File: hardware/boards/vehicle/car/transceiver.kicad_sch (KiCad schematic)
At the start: 0 parts

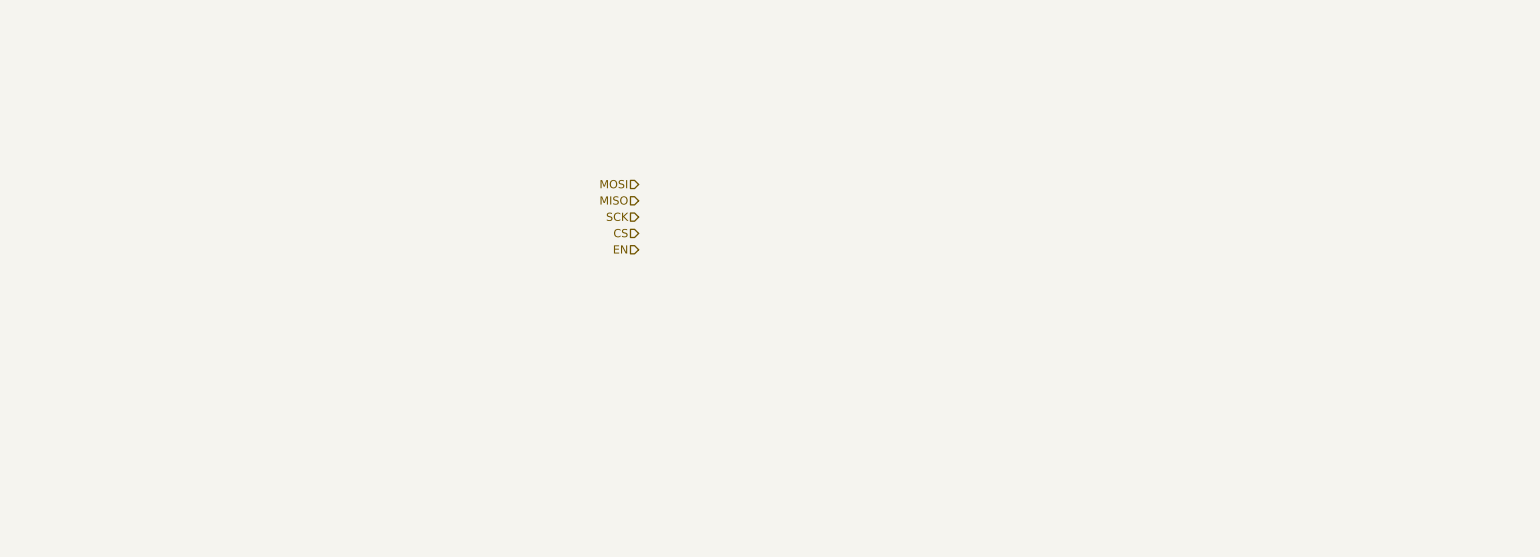
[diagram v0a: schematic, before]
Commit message: car schematic
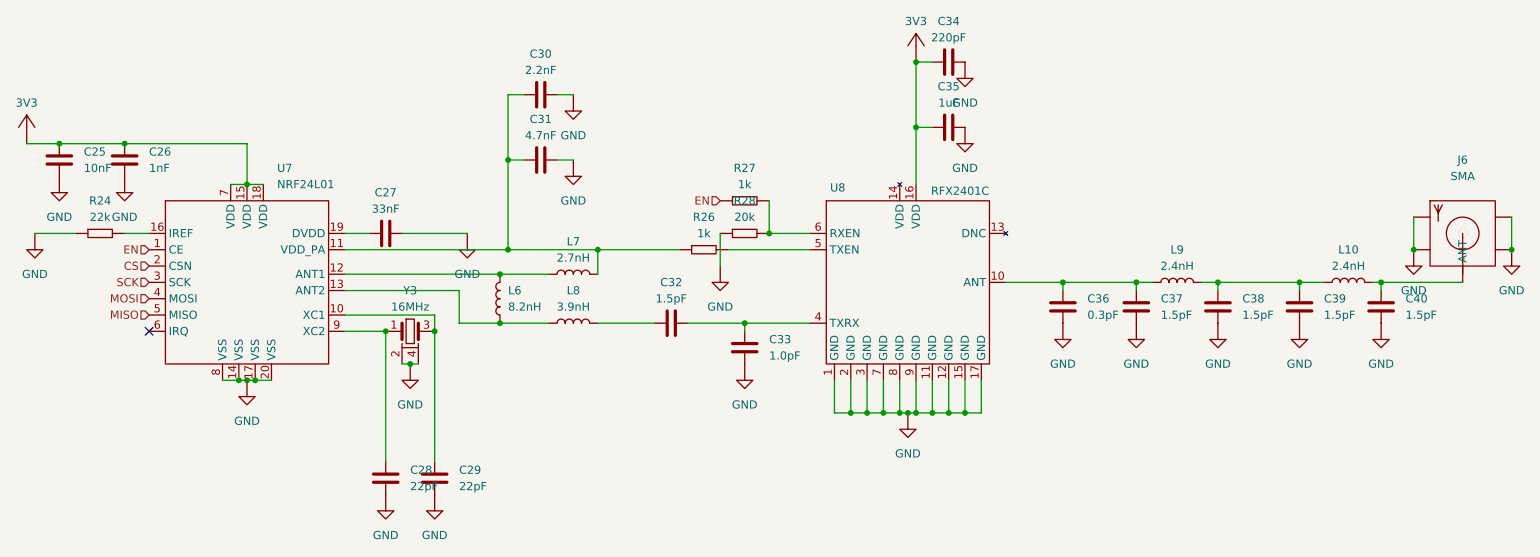
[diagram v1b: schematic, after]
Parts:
- added C25: 10nF, common:C_0603, symbol common:Capacitor
- added C26: 1nF, common:C_0603, symbol common:Capacitor
- added C27: 33nF, common:C_0603, symbol common:Capacitor
- added C28, C29: 22pF, common:C_0603, symbol common:Capacitor
- added C30: 2.2nF, common:C_0603, symbol common:Capacitor
- added C31: 4.7nF, common:C_0603, symbol common:Capacitor
- added C32, C37, C38, C39, C40: 1.5pF, common:C_0603, symbol common:Capacitor
- added C33: 1.0pF, common:C_0603, symbol common:Capacitor
- added C34: 220pF, common:C_0603, symbol common:Capacitor
- added C35: 1uF, common:C_0603, symbol common:Capacitor
- added C36: 0.3pF, common:C_0603, symbol common:Capacitor
- added J6: SMA, connector:SMA, symbol connector:SMA
- added L10, L9: 2.4nH, common:L_0603, symbol common:Inductor
- added L6: 8.2nH, common:L_0603, symbol common:Inductor
- added L7: 2.7nH, common:L_0603, symbol common:Inductor
- added L8: 3.9nH, common:L_0603, symbol common:Inductor
- added R24: 22k, common:R_0603, symbol common:Resistor
- added R26, R27: 1k, common:R_0603, symbol common:Resistor
- added R28: 20k, common:R_0603, symbol common:Resistor
- added U7: NRF24L01, transceiver:NRF24L01_QFN20, symbol transceiver:NRF24L01
- added U8: RFX2401C, transceiver:RFX2401C_QFN16, symbol transceiver:RFX2401C
- added Y3: 16MHz, common:Crystal_3225, symbol common:Crystal_4Pins
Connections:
- net CS: now also U7.2 (CSN)
- net EN: now also R27.1, U7.1 (CE)
- net MISO: now also U7.5 (MISO)
- net MOSI: now also U7.4 (MOSI)
- net SCK: now also U7.3 (SCK)
- new net: C30.1, C31.1, L7.2, R26.1, U7.11 (VDD_PA)
- new net: C29.2, U7.10 (XC1), Y3.3
- new net: L6.2, L7.1, U7.12 (ANT1)
- new net: L6.1, L8.1, U7.13 (ANT2)
- new net: R24.2, U7.16 (IREF)
- new net: C27.1, U7.19 (DVDD)
- new net: C28.2, U7.9 (XC2), Y3.1
- new net: R26.2, U8.5 (TXEN)
- new net: C32.2, C33.2, U8.4 (TXRX)
- new net: C32.1, L8.2
- new net: C38.2, C39.2, L10.1, L9.2
- new net: C36.2, C37.2, L9.1, U8.10 (ANT)
- new net: R27.2, R28.2, U8.6 (RXEN)
- new net: C40.2, J6.1 (ANT), L10.2
- new net 3V3: C25.2, C26.2, C34.1, C35.1, U7.15 (VDD), U7.18 (VDD), U7.7 (VDD), U8.16 (VDD)
- new net GND: C25.1, C26.1, C27.2, C28.1, C29.1, C30.2, C31.2, C33.1, C34.2, C35.2, C36.1, C37.1, C38.1, C39.1, C40.1, J6.2, J6.3, J6.4, J6.5, R24.1, R28.1, U7.14 (VSS), U7.17 (VSS), U7.20 (VSS), U7.8 (VSS), U8.1 (GND), U8.11 (GND), U8.12 (GND), U8.15 (GND), U8.17 (GND), U8.2 (GND), U8.3 (GND), U8.7 (GND), U8.8 (GND), U8.9 (GND), Y3.2 (GND), Y3.4 (GND)
- no-connect marks 0 -> 1
